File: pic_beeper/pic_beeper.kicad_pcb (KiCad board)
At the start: 2 copper layers, 33 x 19.5 mm, 13 parts, among them J1 Conn_01x06, J2 Conn_01x02_Male, J3 Conn_01x02_Female, SW1 SW_SPDT, U1 PIC12F752

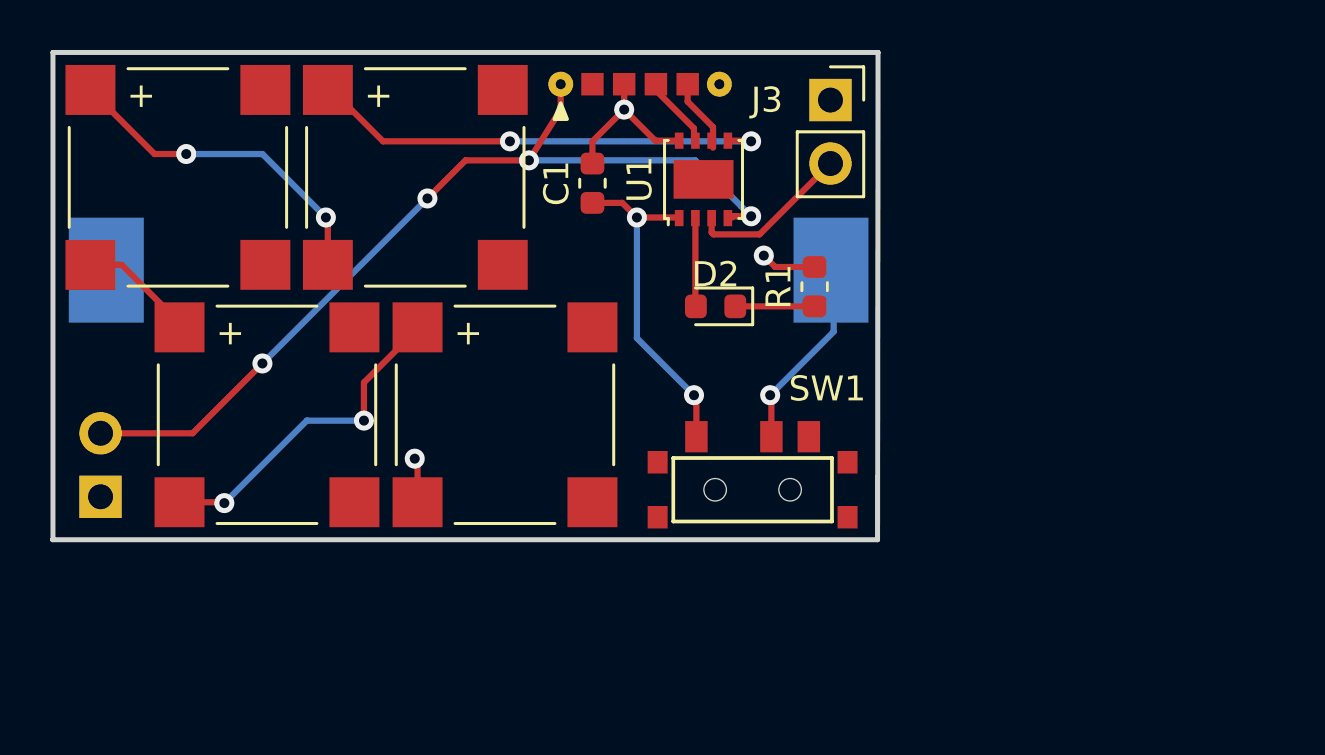
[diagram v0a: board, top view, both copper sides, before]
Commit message: Make hardware v2.0
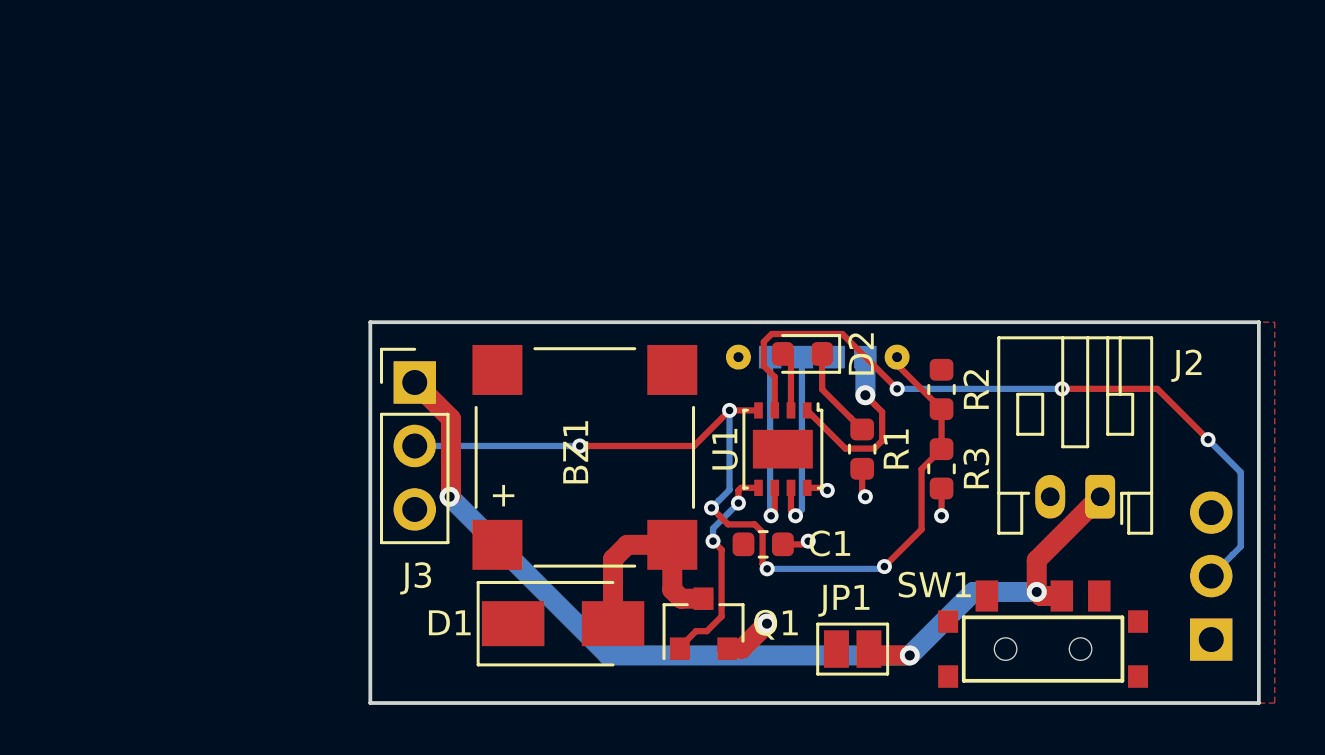
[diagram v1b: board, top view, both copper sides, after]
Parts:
- removed BT1: CR2032, lib_fp:BatteryHolder_Q&J-CR2032-BS-6-1
- removed BZ2, BZ3, BZ4: 16R, Buzzer_Beeper:PUIAudio_SMT_0825_S_4_R
- added D1: 40V 5A, Diode_SMD:D_SMA, F.Cu at (20.4, 22.9)
- added G***: LOGO, lib_fp:bird_with_pants_small_flipped, B.Cu at (20.2, 18.4)
- added G***: LOGO, lib_fp:bird_with_pants_small, B.Cu at (24.0, 18.4)
- added J4: Conn_01x03_Female, Connector_PinSocket_2.54mm:PinSocket_1x03_P2.54mm_Vertical, B.Cu at (46.4, 23.5)
- added JP1: Open Jumper, Jumper:SolderJumper-2_P1.3mm_Open_Pad1.0x1.5mm, F.Cu at (32.0, 23.9)
- added Q1: BSS138, Package_TO_SOT_SMD:SOT-23, F.Cu at (26.0, 22.9)
- added R2: 10k, Resistor_SMD:R_0603_1608Metric, F.Cu at (35.6, 13.5)
- added R3: DNP, Resistor_SMD:R_0603_1608Metric, F.Cu at (35.6, 16.7)
- J1: moved to B.Cu
- J2: value Conn_01x02_Male -> JST_PH_01x02_Male_RightAngle; footprint Connector_PinHeader_2.54mm:PinHeader_1x02_P2.54mm_Vertical -> Connector_JST:JST_PH_S2B-PH-K_1x02_P2.00mm_Horizontal; moved to F.Cu
- J3: value Conn_01x02_Female -> Conn_01x03_Male; footprint Connector_PinSocket_2.54mm:PinSocket_1x02_P2.54mm_Vertical -> Connector_PinHeader_2.54mm:PinHeader_1x03_P2.54mm_Vertical
- R1: value 140R -> 680R
- moved J2 40.0 mm to (41.9, 17.8), turned to 180 degrees
- moved J3 20.1 mm to (14.5, 13.2)
- moved C1 16.0 mm to (28.4, 19.7), turned to 0 degrees
- moved SW1 13.3 mm to (39.6, 23.9)
- moved BZ1 13.1 mm to (21.3, 16.2), turned to 90 degrees
- moved J1 12.6 mm to (30.2, 12.2), turned to 180 degrees
- moved U1 11.3 mm to (29.2, 15.9), turned to 270 degrees
- moved R1 6.78 mm to (32.4, 15.9), turned to 270 degrees
- moved D2 3.97 mm to (30.0, 12.1)
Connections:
- BZ1 pad 1: /BUZZER -> +BATT
- J1 pad 6: Net-(J1-Pad6) -> (no net)
- J2 pad 1: -BATT -> /BATT_SWITCH
- J2 pad 2: /VPP -> -BATT
- J3 pad 1: -BATT -> /BATT_SWITCH
- J3 pad 2: /SLAVE_RESET -> /VPP
- SW1 pad 2: Net-(BT1-Pad1) -> /BATT_SWITCH
- SW1 pad 3: Net-(SW1-Pad3) -> (no net)
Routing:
- net /BATT_SWITCH: track 0.00 -> 40.0 mm, vias 0 -> 3
- net /SLAVE_RESET: track 6.71 -> 29.1 mm, vias 0 -> 3
- net Net-(BZ3-Pad2): track 13.2 -> 0.00 mm, vias 2 -> 0
- net /BUZZER: track 18.5 -> 8.69 mm
- net Net-(BT1-Pad1): track 7.56 -> 0.00 mm, vias 1 -> 0
- net +BATT: track 13.3 -> 7.38 mm, vias 2 -> 1
- net Net-(BZ1-Pad2): track 13.4 -> 8.39 mm, vias 2 -> 0
- net /ICSPDAT: track 2.92 -> 7.65 mm, vias 0 -> 1
- net /ICSPCLK: track 2.96 -> 7.54 mm, vias 0 -> 1
- net Net-(BZ2-Pad2): track 4.53 -> 0.00 mm
- net -BATT: track 10.4 -> 6.18 mm, vias 3 -> 5
- net /VPP: track 35.7 -> 37.4 mm, vias 4 -> 5
- net Net-(D2-Pad2): track 3.47 -> 2.39 mm
- net Net-(D2-Pad1): track 3.18 -> 3.69 mm
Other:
- board size 33 x 19.5 mm -> 35.6 x 15.2 mm
- board text added: "Pic Beeper v2.0 For my favorite human."
- board text removed: "v2.1"
